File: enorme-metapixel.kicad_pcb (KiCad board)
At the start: 2 copper layers, 75 x 75 mm, 42 parts, among them J1 VIN, J2 STRIP_0, J3 STRIP_1, J4 STRIP_2, J5 UART, Q1 SSM3K329R, Q2 SSM3K329R, Q3 SSM3K329R, Q4 SSM3K329R, Q5 SSM3K329R, Q6 SSM3K329R, Q7 SSM3K329R, Q8 SSM3K329R, Q9 SSM3K329R, SW1 SW_RESET, SW2 SW_BOOT, U1 BD33FC0FP, U2 ESP32-WROOM-32

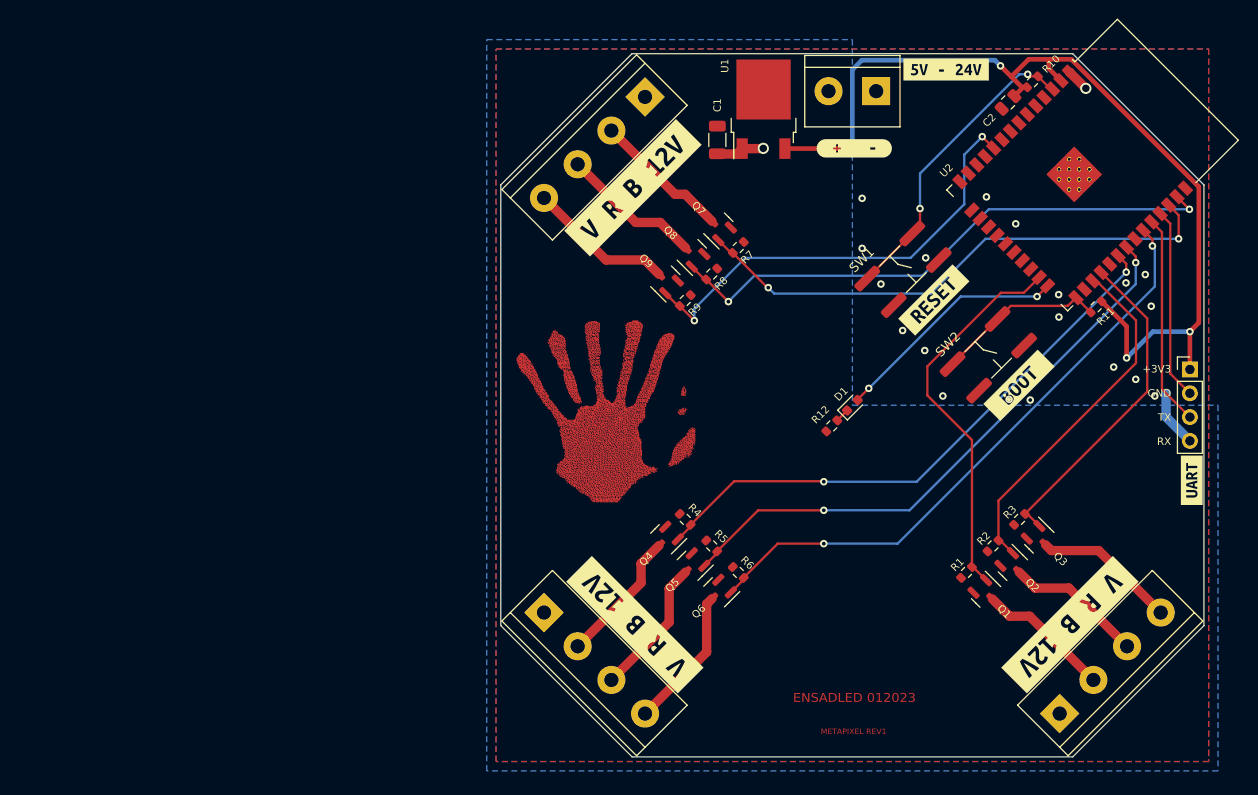
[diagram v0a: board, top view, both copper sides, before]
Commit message: Rev 2
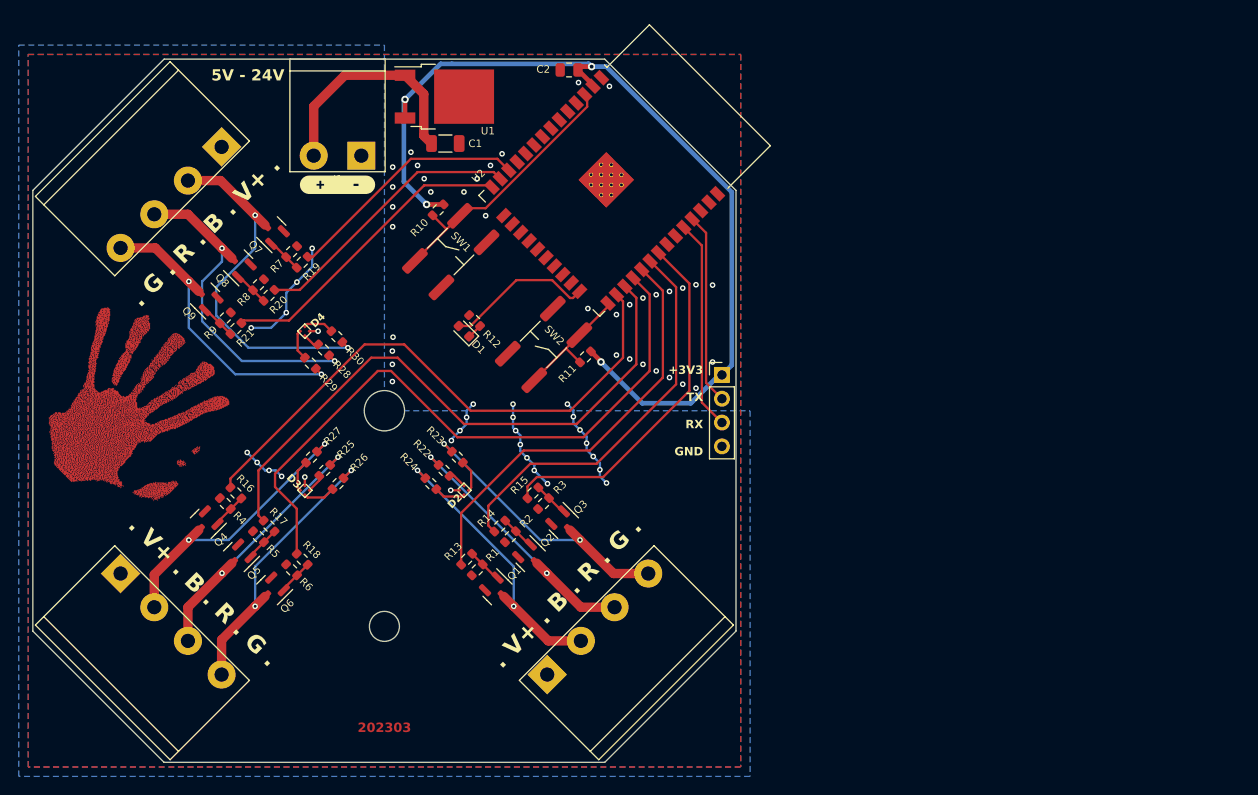
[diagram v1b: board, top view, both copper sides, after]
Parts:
- removed kibuzzard-63B86E19: G***, kibuzzard-63B86E19
- removed kibuzzard-63B86EB9 (x3): G***, kibuzzard-63B86EB9
- removed kibuzzard-63B86F04: G***, kibuzzard-63B86F04
- removed kibuzzard-63B89CDD: G***, kibuzzard-63B89CDD
- removed kibuzzard-63B89D08: G***, kibuzzard-63B89D08
- added D2: Ch.0, ENSADLED:ARGB_0404, F.Cu at (176.1, 106.6)
- added D3: Ch.1, ENSADLED:ARGB_0404, F.Cu at (159.1, 106.6)
- added D4: Ch.2, ENSADLED:ARGB_0404, F.Cu at (159.1, 89.6)
- added H1: M4, MountingHole:MountingHole_4.3mm_M4, F.Cu at (167.6, 98.1)
- added H2: PEG, MountingHole:MountingHole_3.2mm_M3, F.Cu at (167.6, 121.1)
- added R13: 1k, Resistor_SMD:R_0603_1608Metric, F.Cu at (176.4, 113.9)
- added R14: 1k, Resistor_SMD:R_0603_1608Metric, F.Cu at (179.9, 110.4)
- added R15: 1k, Resistor_SMD:R_0603_1608Metric, F.Cu at (183.4, 106.9)
- added R16: 1k, Resistor_SMD:R_0603_1608Metric, F.Cu at (151.8, 106.9)
- added R17: 1k, Resistor_SMD:R_0603_1608Metric, F.Cu at (155.3, 110.4)
- added R18: 1k, Resistor_SMD:R_0603_1608Metric, F.Cu at (158.8, 113.9)
- added R19: 1k, Resistor_SMD:R_0603_1608Metric, F.Cu at (158.8, 82.2)
- added R20: 1k, Resistor_SMD:R_0603_1608Metric, F.Cu at (155.3, 85.8)
- added R21: 1k, Resistor_SMD:R_0603_1608Metric, F.Cu at (151.8, 89.3)
- added R22: 3.3k, Resistor_SMD:R_0603_1608Metric, F.Cu at (174.0, 104.4)
- added R23: 3.3k, Resistor_SMD:R_0603_1608Metric, F.Cu at (175.4, 103.0)
- added R24: 3.3k, Resistor_SMD:R_0603_1608Metric, F.Cu at (172.5, 105.9)
- added R25: 3.3k, Resistor_SMD:R_0603_1608Metric, F.Cu at (161.2, 104.4)
- added R26: 3.3k, Resistor_SMD:R_0603_1608Metric, F.Cu at (162.6, 105.9)
- added R27: 3.3k, Resistor_SMD:R_0603_1608Metric, F.Cu at (159.8, 103.0)
- added R28: 3.3k, Resistor_SMD:R_0603_1608Metric, F.Cu at (161.1, 91.6)
- added R29: 3.3k, Resistor_SMD:R_0603_1608Metric, F.Cu at (159.7, 93.0)
- added R30: 3.3k, Resistor_SMD:R_0603_1608Metric, F.Cu at (162.5, 90.2)
- J1: footprint TerminalBlock:TerminalBlock_bornier-2_P5.08mm -> ENSADLED:fiche_bornier-2_P5.08mm
- J2, J3, J4: footprint TerminalBlock:TerminalBlock_bornier-4_P5.08mm -> ENSADLED:fiche-bornier-4_P5.08mm
- R1, R2, R3, R4, R5, R6, R7, R8, R9: value 10k -> 100k
- moved R10 64.8 mm to (173.3, 76.7), turned to -135 degrees
- moved J1 57.9 mm to (162.6, 70.9)
- moved kibuzzard-63B86E3D 55.2 mm to (162.6, 74.0)
- moved R11 54.7 mm to (189.0, 92.3)
- moved R1 52.2 mm to (177.5, 115.1)
- moved Q1 52.1 mm to (179.7, 117.2)
- moved J4 51.7 mm to (144.8, 75.3)
- moved R2 51.5 mm to (181.0, 111.5)
- moved Q2 51.4 mm to (183.2, 113.7)
- moved G*** 51.4 mm to (139.9, 98.3), turned to -45 degrees
- moved R3 50.8 mm to (184.6, 108.0)
- moved Q3 50.7 mm to (186.7, 110.1)
- moved J2 50.2 mm to (190.3, 120.8)
- moved J5 49.9 mm to (203.6, 94.3)
- moved U2 49.9 mm to (191.1, 74.6)
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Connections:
- Q1 pad 1: /IO15 -> Net-(Q1-G)
- Q2 pad 1: /IO16 -> Net-(Q2-G)
- Q3 pad 1: /IO17 -> Net-(Q3-G)
- Q4 pad 1: /IO18 -> Net-(Q4-G)
- Q5 pad 1: /IO19 -> Net-(Q5-G)
- Q6 pad 1: /IO21 -> Net-(Q6-G)
- Q7 pad 1: /IO22 -> Net-(Q7-G)
- Q8 pad 1: /IO23 -> Net-(Q8-G)
- Q9 pad 1: /IO25 -> Net-(Q9-G)
- R1 pad 1: /IO15 -> Net-(Q1-G)
- R2 pad 1: /IO16 -> Net-(Q2-G)
- R3 pad 1: /IO17 -> Net-(Q3-G)
- R4 pad 1: /IO18 -> Net-(Q4-G)
- R5 pad 1: /IO19 -> Net-(Q5-G)
- R6 pad 1: /IO21 -> Net-(Q6-G)
- R7 pad 1: /IO22 -> Net-(Q7-G)
- R8 pad 1: /IO23 -> Net-(Q8-G)
- R9 pad 1: /IO25 -> Net-(Q9-G)
- U2 pad 10: /IO25 -> unconnected-(U2-IO25-Pad10)
- U2 pad 12: unconnected-(U2-Pad12) -> /ledc6
- U2 pad 13: unconnected-(U2-Pad13) -> /ledc7
- U2 pad 14: unconnected-(U2-Pad14) -> /ledc8
- U2 pad 23: /IO15 -> unconnected-(U2-IO15-Pad23)
- U2 pad 26: unconnected-(U2-Pad26) -> /ledc3
- U2 pad 27: /IO16 -> /ledc4
- U2 pad 28: /IO17 -> /ledc5
- U2 pad 29: unconnected-(U2-Pad29) -> /ledc0
- U2 pad 30: /IO18 -> /ledc1
- U2 pad 31: /IO19 -> /ledc2
- U2 pad 33: /IO21 -> unconnected-(U2-IO21-Pad33)
- U2 pad 36: /IO22 -> unconnected-(U2-IO22-Pad36)
- U2 pad 37: /IO23 -> unconnected-(U2-IO23-Pad37)
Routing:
- net /ledc5: track 0.00 -> 70.5 mm
- net /IO21: track 65.3 -> 0.00 mm, vias 2 -> 0
- net /ledc4: track 0.00 -> 65.3 mm
- net /IO19: track 62.9 -> 0.00 mm, vias 2 -> 0
- net /IO18: track 61.9 -> 0.00 mm, vias 2 -> 0
- net /ledc3: track 0.00 -> 61.0 mm
- net /IO23: track 60.6 -> 0.00 mm, vias 2 -> 0
- net /IO22: track 57.9 -> 0.00 mm, vias 2 -> 0
- net /IO25: track 48.7 -> 0.00 mm, vias 2 -> 0
- net /ledc0: track 0.00 -> 45.5 mm
- net /ledc1: track 0.00 -> 42.7 mm
- net /IO15: track 41.3 -> 0.00 mm
- net /ledc2: track 0.00 -> 38.9 mm
- net /IO16: track 38.0 -> 0.00 mm
- net /IO17: track 35.3 -> 0.00 mm
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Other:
- board text added: "+3V3 TX RX GND"
- board text added: ". G . R . B . V+ ."
- board text added: ". V+ . B . R . G ."
- board text added: "202303"
- board text added: "5V - 24V"
- board text added: "MetaPixel Rev2"
- board text removed: "+3V3 GND TX RX"
- board text removed: "ENSADLED 012023"
- board text removed: "METAPIXEL REV1"
